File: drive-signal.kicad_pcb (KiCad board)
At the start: 2 copper layers, 43.2 x 71.6 mm, 29 parts, among them J1 Conn_01x03_Pin, J10 Conn_01x04_Pin, J11 Conn_01x04_Pin, J2 Conn_01x03_Pin, J3 Conn_01x03_Pin, J4 Conn_01x03_Pin, J5 JETSON, J6 IMU, J7 Conn_01x02_Pin, J8 Conn_01x04_Pin, J9 Conn_01x04_Pin, U1 STM32F4

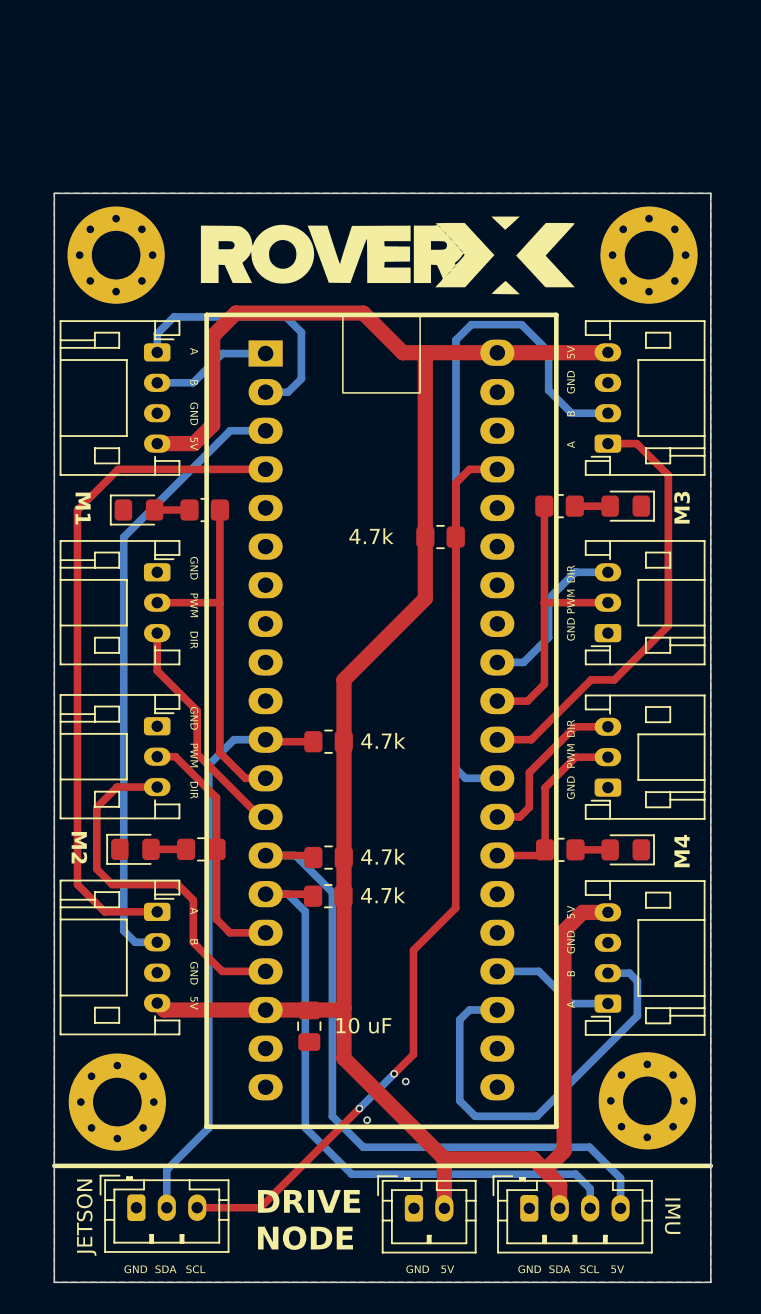
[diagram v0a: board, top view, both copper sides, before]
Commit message: done placement
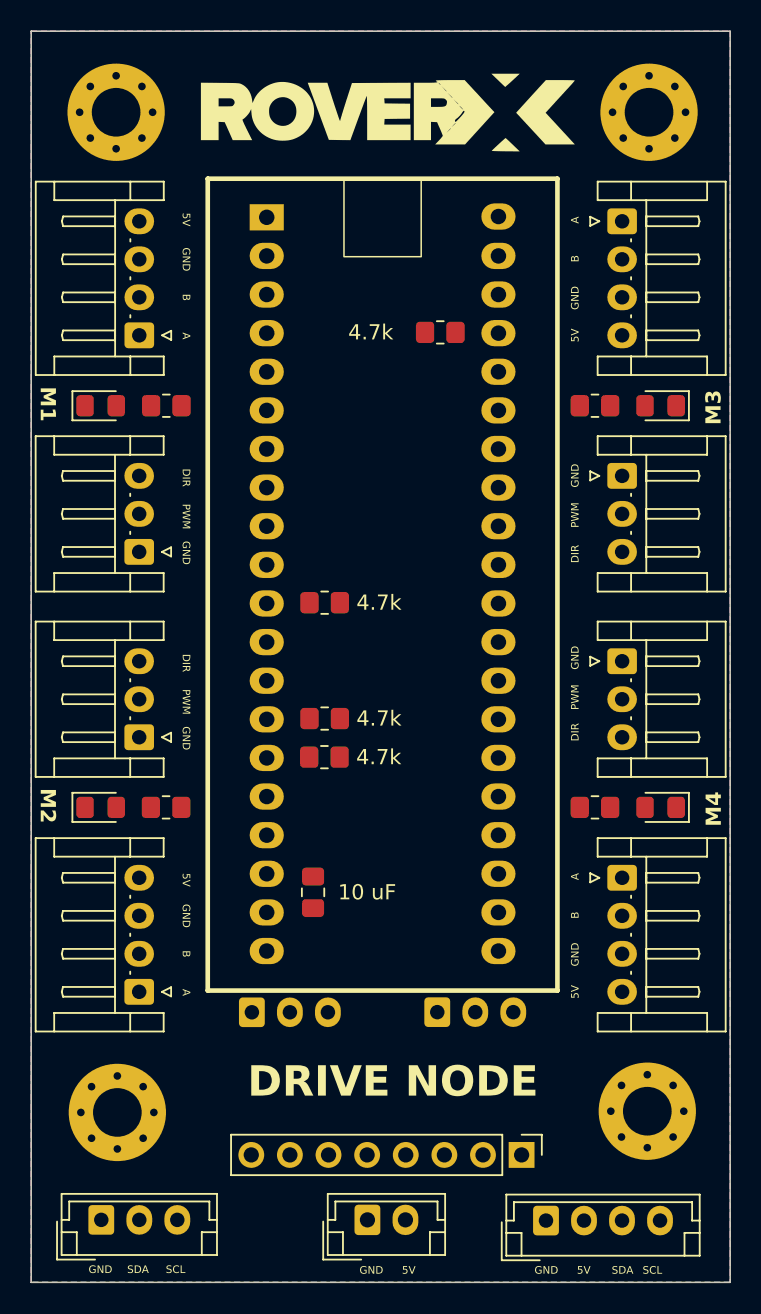
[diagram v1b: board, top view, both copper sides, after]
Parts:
- added J12: IMU, Connector_PinHeader_2.54mm:PinHeader_1x08_P2.54mm_Vertical, F.Cu at (77.5, 89.4)
- added J13: I2C2 P1, Connector_JST:JST_EH_S3B-EH_1x03_P2.50mm_Horizontal, B.Cu at (59.7, 80.0)
- added J14: I2C2 P2, Connector_JST:JST_EH_S3B-EH_1x03_P2.50mm_Horizontal, B.Cu at (71.9, 80.0)
- J1, J2, J3, J4: footprint Connector_JST:JST_PH_S3B-PH-K_1x03_P2.00mm_Horizontal -> Connector_JST:JST_EH_S3B-EH_1x03_P2.50mm_Horizontal
- J10, J11, J8, J9: footprint Connector_JST:JST_PH_S4B-PH-K_1x04_P2.00mm_Horizontal -> Connector_JST:JST_EH_S4B-EH_1x04_P2.50mm_Horizontal
- J5: footprint Connector_JST:JST_PH_B3B-PH-K_1x03_P2.00mm_Vertical -> Connector_JST:JST_EH_B3B-EH-A_1x03_P2.50mm_Vertical
- J6: footprint Connector_JST:JST_PH_B4B-PH-K_1x04_P2.00mm_Vertical -> Connector_JST:JST_EH_B4B-EH-A_1x04_P2.50mm_Vertical
- J7: footprint Connector_JST:JST_PH_B2B-PH-K_1x02_P2.00mm_Vertical -> Connector_JST:JST_EH_B2B-EH-A_1x02_P2.50mm_Vertical
- moved J11 14.7 mm to (84.1, 28.0), turned to -90 degrees
- moved R4 13.5 mm to (72.1, 35.3)
- moved J4 10.4 mm to (84.1, 44.7), turned to -90 degrees
- moved H1 9.40 mm to (85.9, 20.8)
- moved H2 9.40 mm to (50.8, 20.8)
- moved R1 9.15 mm to (64.5, 63.2)
- moved R3 9.15 mm to (64.5, 53.1)
- moved R2 9.15 mm to (64.5, 60.7)
- moved U1 8.96 mm to (60.7, 27.8)
- moved C1 8.81 mm to (63.8, 72.1)
- moved J3 8.36 mm to (84.1, 56.9), turned to -90 degrees
- moved J10 8.33 mm to (84.1, 71.2), turned to -90 degrees
- moved D2 7.31 mm to (49.8, 40.1)
- moved R6 7.31 mm to (54.1, 40.1)
- moved R8 7.00 mm to (82.3, 40.1)
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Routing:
- net +5V: track 141.0 -> 0.00 mm
- net I2C2_J_SCL: track 60.2 -> 0.00 mm, vias 2 -> 0
- net I2C1_I_SCL: track 45.9 -> 0.00 mm
- net RB_B: track 45.5 -> 0.00 mm
- net LB_A: track 44.1 -> 0.00 mm
- net I2C1_I_SDA: track 42.2 -> 0.00 mm
- net LB_B: track 40.6 -> 0.00 mm
- net I2C2_J_SDA: track 37.9 -> 0.00 mm
- net RB_A: track 29.1 -> 0.00 mm
- net RF_B: track 27.4 -> 0.00 mm
- net DIR_LB: track 24.1 -> 0.00 mm
- net PWM_LF: track 23.8 -> 0.00 mm
- net PWM_RB: track 19.4 -> 0.00 mm
- net LF_A: track 17.4 -> 0.00 mm
- net PWM_LB: track 16.6 -> 0.00 mm
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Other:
- board size 43.2 x 71.6 mm -> 46 x 82.3 mm
